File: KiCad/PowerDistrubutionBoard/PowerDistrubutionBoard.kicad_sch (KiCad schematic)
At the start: 10 parts, among them J1 BEC, J2 RS_OUT, J4 R-, J5 R+, J6 RS, T1 PWR_D1, T2 PWR_D2, T3 PWR_IN, T4 PWR_W

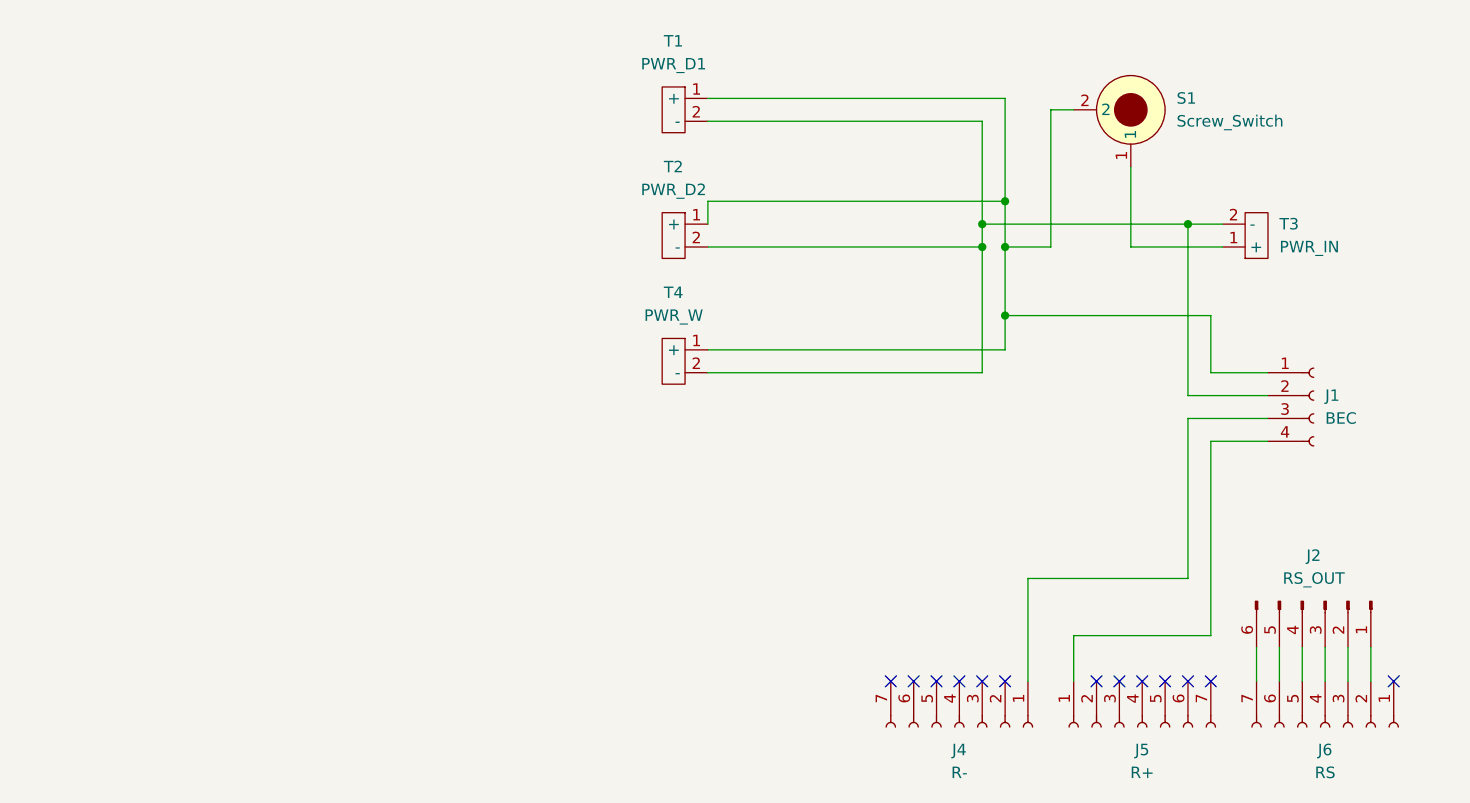
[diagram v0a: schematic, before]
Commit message: new stuff
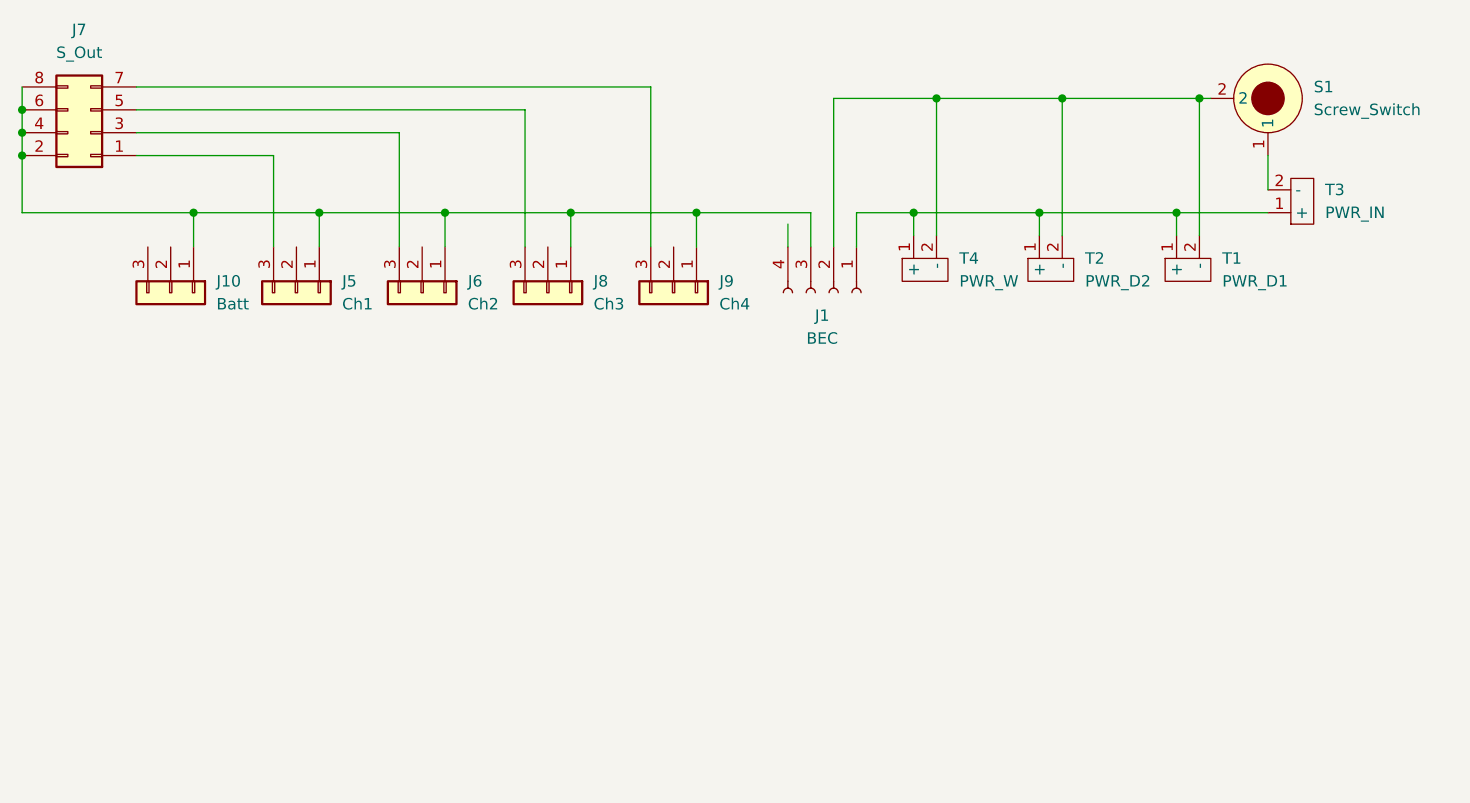
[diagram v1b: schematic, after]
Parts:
- removed J1: BEC, Connector_PinHeader_2.00mm:PinHeader_1x04_P2.00mm_Vertical, symbol Connector:Conn_01x04_Female
- removed J2: RS_OUT, Connector_PinHeader_2.54mm:PinHeader_1x06_P2.54mm_Vertical, symbol Connector:Conn_01x06_Male
- removed J4: R-, Connector_PinHeader_2.54mm:PinHeader_1x07_P2.54mm_Vertical, symbol Connector:Conn_01x07_Female
- removed J5: R+, Connector_PinHeader_2.54mm:PinHeader_1x07_P2.54mm_Vertical, symbol Connector:Conn_01x07_Female
- removed J6: RS, Connector_PinHeader_2.54mm:PinHeader_1x07_P2.54mm_Vertical, symbol Connector:Conn_01x07_Female
- added J1: BEC, Connector_PinHeader_2.54mm:PinHeader_1x04_P2.54mm_Vertical, symbol Connector:Conn_01x04_Socket
- added J10: Batt, Connector_PinHeader_2.54mm:PinHeader_1x03_P2.54mm_Vertical, symbol Connector_Generic:Conn_01x03
- added J5: Ch1, Connector_PinHeader_2.54mm:PinHeader_1x03_P2.54mm_Vertical, symbol Connector_Generic:Conn_01x03
- added J6: Ch2, Connector_PinHeader_2.54mm:PinHeader_1x03_P2.54mm_Vertical, symbol Connector_Generic:Conn_01x03
- added J7: S_Out, Connector_PinHeader_2.54mm:PinHeader_2x04_P2.54mm_Horizontal, symbol Connector_Generic:Conn_02x04_Odd_Even
- added J8: Ch3, Connector_PinHeader_2.54mm:PinHeader_1x03_P2.54mm_Vertical, symbol Connector_Generic:Conn_01x03
- added J9: Ch4, Connector_PinHeader_2.54mm:PinHeader_1x03_P2.54mm_Vertical, symbol Connector_Generic:Conn_01x03
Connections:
- net at T1.1 (+), T2.1 (+), T4.1 (+): now also T3.1 (+), J1.1 (Pin_1); no longer S1.2
- net at T1.2 (-), T2.2 (-), T4.2 (-): now also S1.2, J1.2 (Pin_2); no longer T3.2 (-)
- net at S1.1: now also T3.2 (-); no longer T3.1 (+)
- new net: J1.3 (Pin_3), J10.1 (Pin_1), J5.1 (Pin_1), J6.1 (Pin_1), J7.2 (Pin_2), J7.4 (Pin_4), J7.6 (Pin_6), J7.8 (Pin_8), J8.1 (Pin_1), J9.1 (Pin_1)
- new net: J7.5 (Pin_5), J8.3 (Pin_3)
- new net: J7.7 (Pin_7), J9.3 (Pin_3)
- new net: J5.3 (Pin_3), J7.1 (Pin_1)
- new net: J6.3 (Pin_3), J7.3 (Pin_3)
- no-connect marks 13 -> 0
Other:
- moved on the sheet: S1, T1, T2, T3, T4
